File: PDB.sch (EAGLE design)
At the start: 77 parts, among them IC1 LM555N

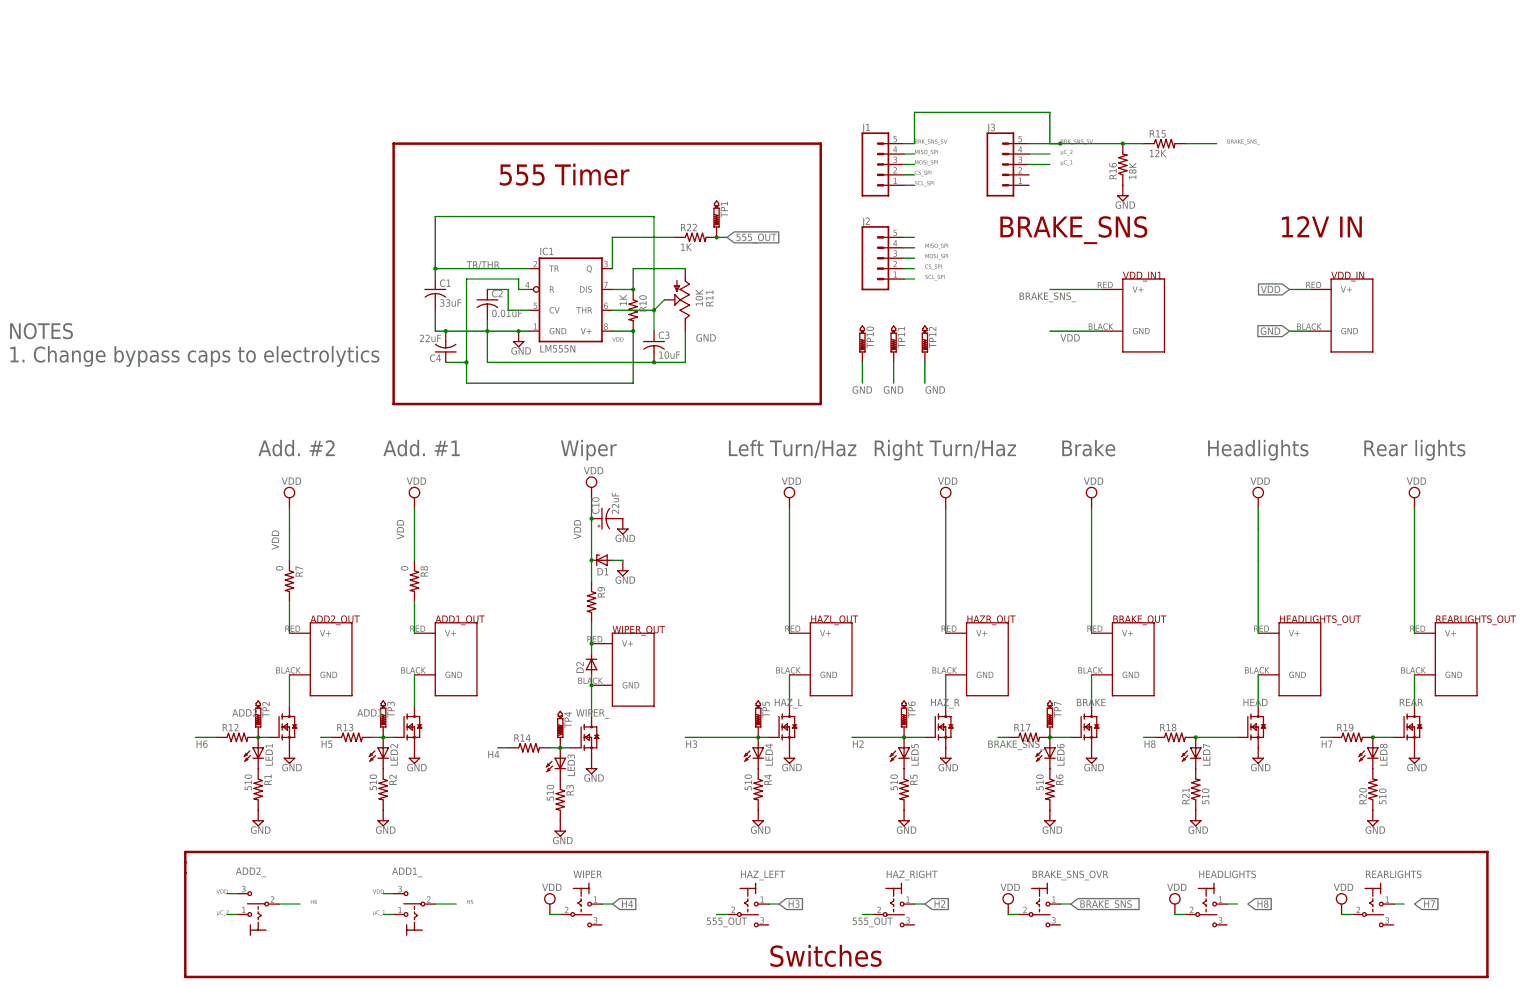
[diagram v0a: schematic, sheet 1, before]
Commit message: added Molex for MC signals
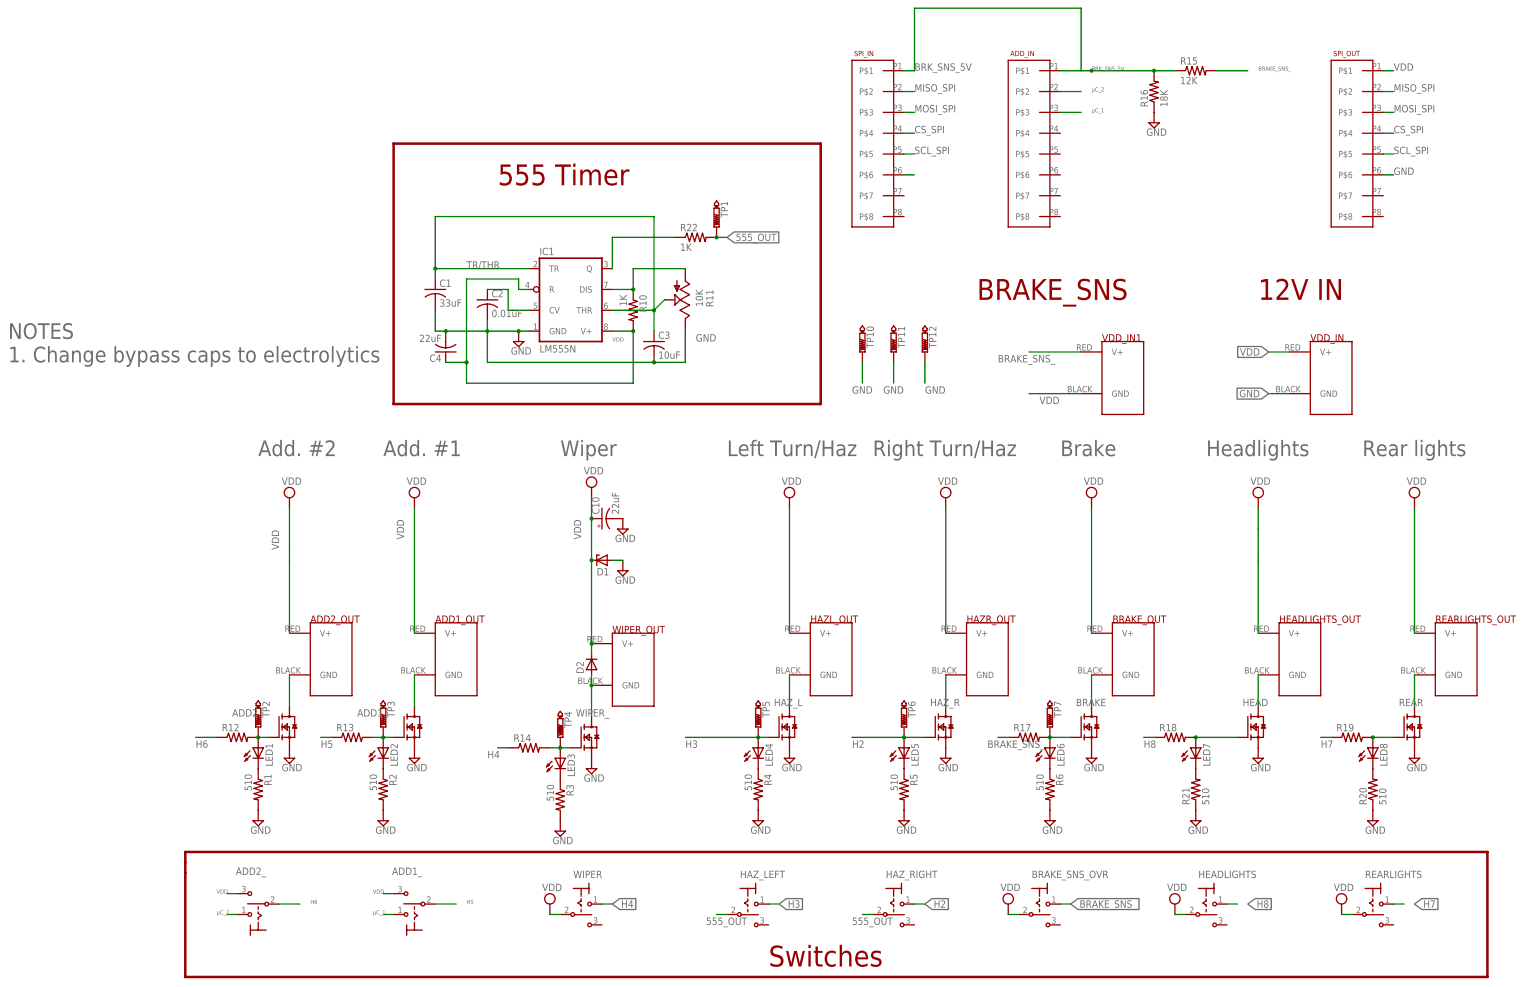
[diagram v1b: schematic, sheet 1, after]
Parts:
- removed J1, J2, J3: (no value), SparkFun-Connectors:CONN_05JST
- removed R7, R8: 0, rcl:R-US_R0805
- removed R9: (no value), rcl:R-US_R0805
- added ADD_IN, SPI_IN, SPI_OUT: 8-PIN-MOLEX-RA-FEMALE, master_library:8-PIN-MOLEX-RA-FEMALE
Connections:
- removed net N$12: J2.5
- removed net N$16: ADD2_OUT.V+, R7.2
- removed net N$20: D2.C, R9.2, WIPER_OUT.V+
- net BRK_SNS_5V: now also ADD_IN.P$1, SPI_IN.P$1; no longer J1.5, J3.5
- net CS_SPI: now also SPI_IN.P$4, SPI_OUT.P$4; no longer J1.2, J2.2
- net GND: now also SPI_OUT.P$6
- net MISO_SPI: now also SPI_IN.P$2, SPI_OUT.P$2; no longer J1.4, J2.4
- net MOSI_SPI: now also SPI_IN.P$3, SPI_OUT.P$3; no longer J1.3, J2.3
- net N$18: now also SPI_IN.P$6; no longer ADD1_OUT.V+, R8.2
- net SCL_SPI: now also SPI_IN.P$5, SPI_OUT.P$5; no longer J1.1, J2.1
- net VDD: now also ADD1_OUT.V+, ADD2_OUT.V+, D2.C, SPI_OUT.P$1, WIPER_OUT.V+; no longer R7.1, R8.1, R9.1
- net µC_1: now also ADD_IN.P$3; no longer J3.3
- net µC_2: now also ADD_IN.P$2; no longer J3.4
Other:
- moved on the sheet: R15, R16, VDD_IN, VDD_IN1
